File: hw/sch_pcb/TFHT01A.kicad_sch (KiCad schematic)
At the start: 24 parts, among them J1 SM04B-GHS-TB, J2 SM04B-GHS-TB, M1 M3, M2 M3, M3 M3, M4 M3, M5 M3, M6 M3, Q1 BC817, U1 SHT31, U3 MIC5504-3.3YM5

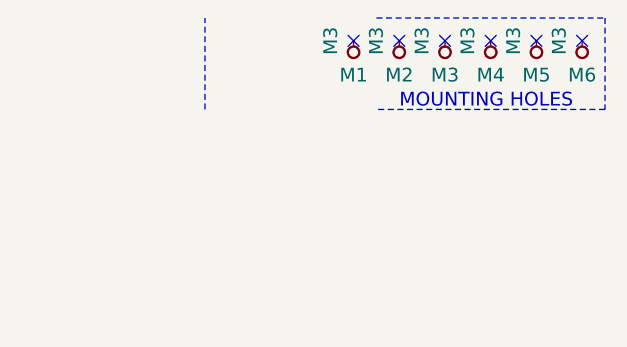
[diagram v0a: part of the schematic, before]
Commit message: Minor graphics improvement.
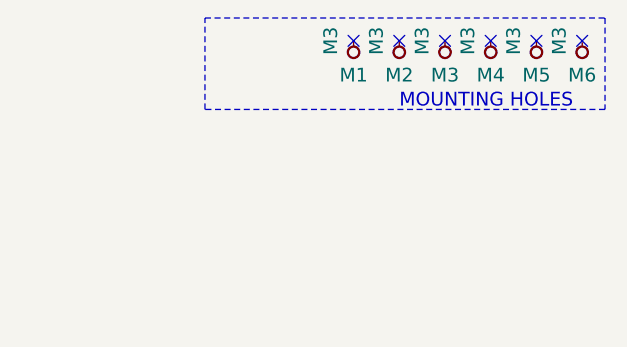
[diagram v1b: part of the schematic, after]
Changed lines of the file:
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@@
     (stroke (width 0) (type solid) (color 0 0 0 0))
   )
-  (polyline (pts (xy 236.22 27.94) (xy 236.22 17.78))
+  (polyline (pts (xy 236.22 17.78) (xy 280.67 17.78))
     (stroke (width 0) (type dash) (color 0 0 0 0))
   )
-  (polyline (pts (xy 255.27 17.78) (xy 280.67 17.78))
+  (polyline (pts (xy 236.22 27.94) (xy 236.22 17.78))
     (stroke (width 0) (type dash) (color 0 0 0 0))
   )
@@
     (stroke (width 0) (type dash) (color 0 0 0 0))
   )
-  (polyline (pts (xy 280.67 27.94) (xy 255.27 27.94))
+  (polyline (pts (xy 280.67 27.94) (xy 236.22 27.94))
     (stroke (width 0) (type dash) (color 0 0 0 0))
   )

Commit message: Edit
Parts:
- D1: UST_ID 604b0326128750769e5b0f93 -> 60879d38128750769ee58e48
- D2: UST_ID (none) -> 5c70984412875079b91f8895
- D3: UST_ID (none) -> 5c70984412875079b91f8896
- Q1: UST_ID (none) -> 5c70984712875079b91f8aec
- R1, R4: UST_ID (none) -> 5c70984512875079b91f8957
- R10, R3: UST_ID 5c70984612875079b91f899f -> 5c70984512875079b91f8962
- R2: UST_ID (none) -> 5c70984512875079b91f8956
- U1: UST_ID (none) -> 5c70984612875079b91f89e4
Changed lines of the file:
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@@
+      (effects (font (size 1.27 1.27)) hide)
+    )
+    (property "UST_ID" "5c70984512875079b91f8957" (id 4) (at 20.32 168.91 0)
       (effects (font (size 1.27 1.27)) hide)
     )
@@
       (effects (font (size 1.27 1.27)) hide)
     )
-    (property "UST_ID" "5c70984612875079b91f899f" (id 5) (at 147.32 87.63 0)
+    (property "UST_ID" "5c70984512875079b91f8962" (id 5) (at 147.32 87.63 0)
       (effects (font (size 1.27 1.27)) hide)
     )
@@
       (effects (font (size 1.27 1.27)) hide)
     )
-    (property "UST_ID" "5c70984612875079b91f899f" (id 5) (at 153.67 87.63 0)
+    (property "UST_ID" "5c70984512875079b91f8962" (id 5) (at 153.67 87.63 0)
       (effects (font (size 1.27 1.27)) hide)
     )
@@
       (effects (font (size 1.27 1.27)) hide)
     )
+    (property "UST_ID" "5c70984512875079b91f8956" (id 4) (at 255.27 144.78 0)
+      (effects (font (size 1.27 1.27)) hide)
+    )
     (pin "1")
     (pin "2")
@@
       (effects (font (size 1.27 1.27)) hide)
     )
+    (property "UST_ID" "5c70984512875079b91f8957" (id 4) (at 269.24 133.35 0)
+      (effects (font (size 1.27 1.27)) hide)
+    )
     (pin "1")
     (pin "2")
@@
       (effects (font (size 1.27 1.27)) hide)
     )
-    (property "UST_ID" "604b0326128750769e5b0f93" (id 5) (at 43.18 175.26 0)
+    (property "UST_ID" "60879d38128750769ee58e48" (id 5) (at 43.18 175.26 0)
       (effects (font (size 1.27 1.27)) hide)
     )
@@
       (effects (font (size 1.27 1.27)) hide)
     )
+    (property "UST_ID" "5c70984412875079b91f8895" (id 4) (at 20.32 177.8 0)
+      (effects (font (size 1.27 1.27)) hide)
+    )
     (pin "1")
     (pin "2")
@@
     )
     (property "Datasheet" "~" (id 3) (at 269.24 123.19 0)
+      (effects (font (size 1.27 1.27)) hide)
+    )
+    (property "UST_ID" "5c70984412875079b91f8896" (id 4) (at 269.24 123.19 0)
       (effects (font (size 1.27 1.27)) hide)
     )
@@
       (effects (font (size 1.27 1.27)) (justify left) hide)
     )
+    (property "UST_ID" "5c70984712875079b91f8aec" (id 4) (at 266.7 144.78 0)
+      (effects (font (size 1.27 1.27)) hide)
+    )
     (pin "1")
     (pin "2")
@@
       (effects (font (size 1.524 1.524)))
     )
-    (pin "1")
+    (property "UST_ID" "5c70984612875079b91f89e4" (id 4) (at 127 102.87 0)
+      (effects (font (size 1.27 1.27)) hide)
+    )
+    (pin "1")
